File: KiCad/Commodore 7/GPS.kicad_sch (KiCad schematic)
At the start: 2 parts, among them U2 NEO-M9N-00B

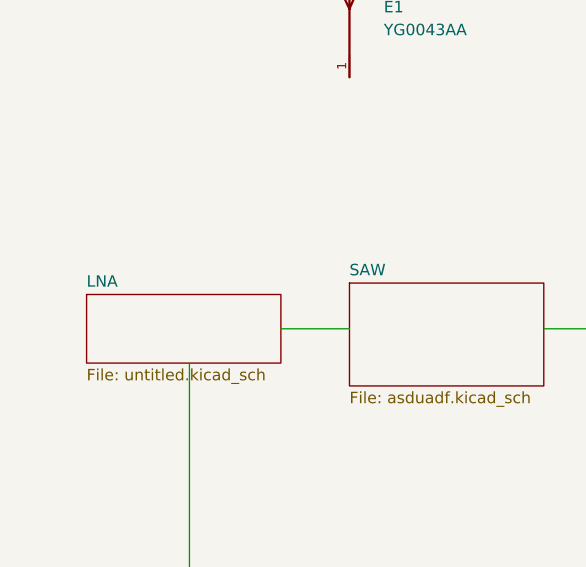
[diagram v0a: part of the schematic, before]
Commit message: hi!!!!!
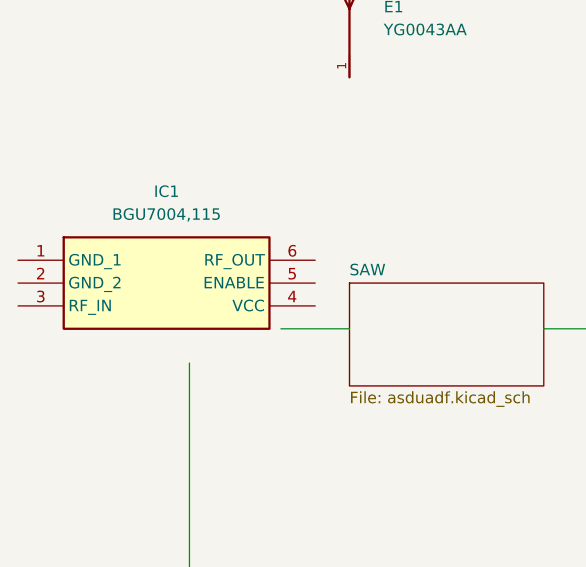
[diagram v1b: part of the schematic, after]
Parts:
- added IC1: BGU7004,115, BGU7004:BGU7004115, symbol BGU7004_115:BGU7004,115
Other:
- removed sheet LNA
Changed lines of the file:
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@@
+	)
+	(symbol
+		(lib_id "BGU7004_115:BGU7004,115")
+		(at 13.97 76.2 0)
+		(unit 1)
+		(exclude_from_sim no)
+		(in_bom yes)
+		(on_board yes)
+		(dnp no)
+		(fields_autoplaced yes)
+		(property "Reference" "IC1"
+			(at 30.48 68.58 0)
+			(effects
+				(font
+					(size 1.27 1.27)
+				)
+			)
+		)
+		(property "Value" "BGU7004,115"
+			(at 30.48 71.12 0)
+			(effects
+				(font
+					(size 1.27 1.27)
+				)
+			)
+		)
+		(property "Footprint" "BGU7004:BGU7004115"
+			(at 43.18 171.12 0)
+			(effects
+				(font
+					(size 1.27 1.27)
+				)
+				(justify left top)
+				(hide yes)
+			)
+		)
+		(property "Datasheet" "https://www.nxp.com/docs/en/data-sheet/BGU7004.pdf"
+			(at 43.18 271.12 0)
+			(effects
+				(font
+					(size 1.27 1.27)
+				)
+				(justify left top)
+				(hide yes)
+			)
+		)
+		(property "Description" "RF Amplifier Low Noise Amplifier"
+			(at 13.97 76.2 0)
+			(effects
+				(font
+					(size 1.27 1.27)
+				)
+				(hide yes)
+			)
+		)
+		(property "Height" "0.5"
+			(at 43.18 471.12 0)
+			(effects
+				(font
+					(size 1.27 1.27)
+				)
+				(justify left top)
+				(hide yes)
+			)
+		)
+		(property "Manufacturer_Name" "NXP"
+			(at 43.18 571.12 0)
+			(effects
+				(font
+					(size 1.27 1.27)
+				)
+				(justify left top)
+				(hide yes)
+			)
+		)
+		(property "Manufacturer_Part_Number" "BGU7004,115"
+			(at 43.18 671.12 0)
+			(effects
+				(font
+					(size 1.27 1.27)
+				)
+				(justify left top)
+				(hide yes)
+			)
+		)
+		(property "Mouser Part Number" "771-BGU7004,115"
+			(at 43.18 771.12 0)
+			(effects
+				(font
+					(size 1.27 1.27)
+				)
+				(justify left top)
+				(hide yes)
+			)
+		)
+		(property "Mouser Price/Stock" "https://www.mouser.co.uk/ProductDetail/NXP-Semiconductors/BGU7004115?qs=vbj%2FKoHZRAjvSA08C7lcmQ%3D%3D"
+			(at 43.18 871.12 0)
+			(effects
+				(font
+					(size 1.27 1.27)
+				)
+				(justify left top)
+				(hide yes)
+			)
+		)
+		(property "Arrow Part Number" ""
+			(at 43.18 971.12 0)
+			(effects
+				(font
+					(size 1.27 1.27)
+				)
+				(justify left top)
+				(hide yes)
+			)
+		)
+		(property "Arrow Price/Stock" ""
+			(at 43.18 1071.12 0)
+			(effects
+				(font
+					(size 1.27 1.27)
+				)
+				(justify left top)
+				(hide yes)
+			)
+		)
+		(pin "6"
+		)
+		(pin "3"
+		)
+		(pin "4"
+		)
+		(pin "2"
+		)
+		(pin "1"
+		)
+		(pin "5"
+		)
+		(instances
+			(project ""
+				(path "/42cf917d-ec14-4557-b98d-6a3f3b8cf25c/bd54c1aa-247c-4340-9de9-44d0c0e040e9"
+					(reference "IC1")
+					(unit 1)
+				)
+			)
+		)
 	)
 	(symbol
@@
 				)
 			)
-		)
-	)
-	(sheet
-		(at 21.59 80.01)
-		(size 21.59 7.62)
-		(exclude_from_sim no)
-		(in_bom yes)
-		(on_board yes)
-		(dnp no)
-		(fields_autoplaced yes)
-		(stroke
-			(width 0.1524)
-			(type solid)
-		)
-		(fill
-			(color 0 0 0 0.0000)
-		)
-		(property "Sheetname" "LNA"
-			(at 21.59 79.2984 0)
-			(effects
-				(font
-					(size 1.27 1.27)
-				)
-				(justify left bottom)
-			)
-		)
-		(property "Sheetfile" "untitled.kicad_sch"
-			(at 21.59 88.2146 0)
-			(effects
-				(font
-					(size 1.27 1.27)
-				)
-				(justify left top)
-			)
-		)
-		(instances
-			(project "Commodore 7"
-				(path "/42cf917d-ec14-4557-b98d-6a3f3b8cf25c/bd54c1aa-247c-4340-9de9-44d0c0e040e9"
-					(page "10")
-				)
-			)
